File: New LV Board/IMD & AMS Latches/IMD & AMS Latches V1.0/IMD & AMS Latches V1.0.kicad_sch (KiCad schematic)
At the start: 21 parts, among them J2 B12B-PH-K-S, K1 A161CS12VDC.64, K2 A161CS12VDC.64, K3 A161CS12VDC.64, K4 A161CS12VDC.64, K5 A161CS12VDC.64, K6 A161CS12VDC.64, SW1 Test Reset IMD, SW2 Test Reset IMD

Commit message: added 3d models to the full part
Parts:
- D1, D2, D5, D6: footprint Diode_THT:D_DO-41_SOD81_P3.81mm_Vertical_AnodeUp -> motorsports:D_DO-41_SOD81_P3.81mm_Vertical_AnodeUp
- K1, K2, K3, K4, K5, K6: footprint Library:RELAY_A161CS12VDC.64 -> motorsports:RELAY_A161CS12VDC.64
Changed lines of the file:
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@@
 			)
 		)
-		(property "Footprint" "Library:RELAY_A161CS12VDC.64"
+		(property "Footprint" "motorsports:RELAY_A161CS12VDC.64"
 			(at 71.12 139.7 0)
 			(effects
@@
 			)
 		)
-		(property "Footprint" "Diode_THT:D_DO-41_SOD81_P3.81mm_Vertical_AnodeUp"
+		(property "Footprint" "motorsports:D_DO-41_SOD81_P3.81mm_Vertical_AnodeUp"
 			(at 133.35 147.32 0)
 			(effects
@@
 			)
 		)
-		(property "Footprint" "Library:RELAY_A161CS12VDC.64"
+		(property "Footprint" "motorsports:RELAY_A161CS12VDC.64"
 			(at 71.12 113.03 0)
 			(effects
@@
 			)
 		)
-		(property "Footprint" "Diode_THT:D_DO-41_SOD81_P3.81mm_Vertical_AnodeUp"
+		(property "Footprint" "motorsports:D_DO-41_SOD81_P3.81mm_Vertical_AnodeUp"
 			(at 50.8 147.32 0)
 			(effects
@@
 			)
 		)
-		(property "Footprint" "Diode_THT:D_DO-41_SOD81_P3.81mm_Vertical_AnodeUp"
+		(property "Footprint" "motorsports:D_DO-41_SOD81_P3.81mm_Vertical_AnodeUp"
 			(at 128.27 147.32 0)
 			(effects
@@
 			)
 		)
-		(property "Footprint" "Diode_THT:D_DO-41_SOD81_P3.81mm_Vertical_AnodeUp"
+		(property "Footprint" "motorsports:D_DO-41_SOD81_P3.81mm_Vertical_AnodeUp"
 			(at 55.88 147.32 0)
 			(effects
@@
 			)
 		)
-		(property "Footprint" "Library:RELAY_A161CS12VDC.64"
+		(property "Footprint" "motorsports:RELAY_A161CS12VDC.64"
 			(at 148.59 139.7 0)
 			(effects
@@
 			)
 		)
-		(property "Footprint" "Library:RELAY_A161CS12VDC.64"
+		(property "Footprint" "motorsports:RELAY_A161CS12VDC.64"
 			(at 148.59 113.03 0)
 			(effects
@@
 			)
 		)
-		(property "Footprint" "Library:RELAY_A161CS12VDC.64"
+		(property "Footprint" "motorsports:RELAY_A161CS12VDC.64"
 			(at 148.59 86.36 0)
 			(effects
@@
 			)
 		)
-		(property "Footprint" "Library:RELAY_A161CS12VDC.64"
+		(property "Footprint" "motorsports:RELAY_A161CS12VDC.64"
 			(at 71.12 86.36 0)
 			(effects

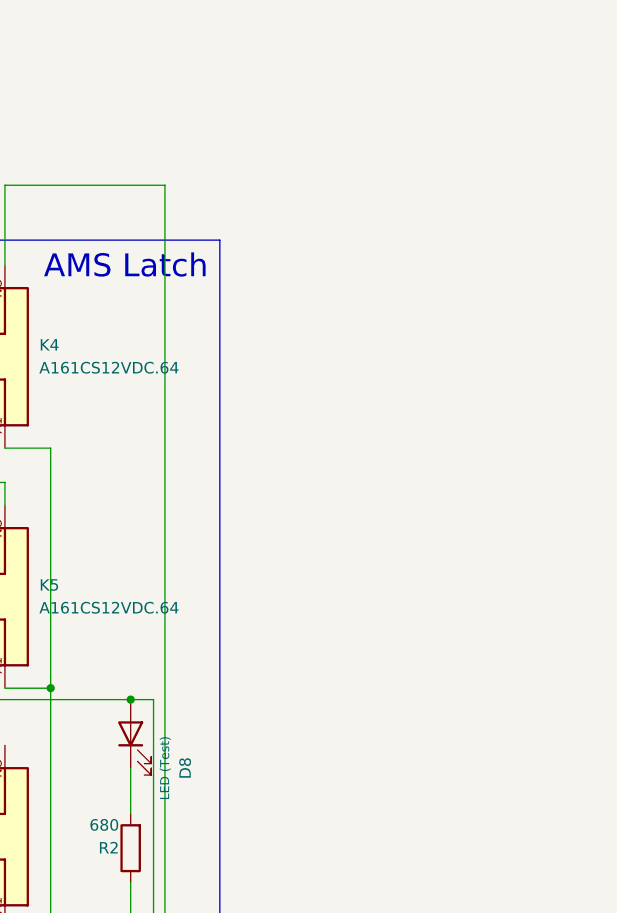
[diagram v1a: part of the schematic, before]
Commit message: changes that can probably be overriden?
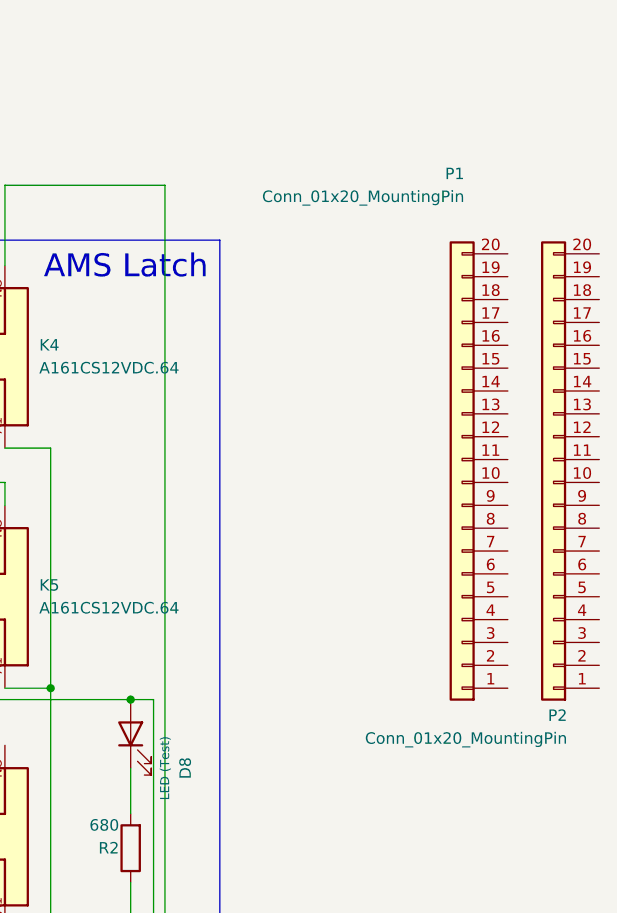
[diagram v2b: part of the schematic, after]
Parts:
- added P1, P2: Conn_01x20_MountingPin, Connector_PinHeader_2.54mm:PinHeader_1x20_P2.54mm_Vertical, symbol Connector_Generic:Conn_01x20
- D1, D2, D5, D6: Part # (none) -> 1N4743A
- D3, D7: Part # (none) -> 1N4001
- K1, K2, K3, K4, K5, K6: MANUFACTURER CIT -> (none); MAXIMUM_PACKAGE_HEIGHT 13.85mm -> (none); PARTREV B -> (none); SNAPEDA_PN A161CS12VDC.64 -> (none); STANDARD Manufacturer Recommendations -> (none)

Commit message: Revert "changes that can probably be overriden?"
This reverts commit 98343f344ad0564068fa41cd25b8ec5d82cca4ea.
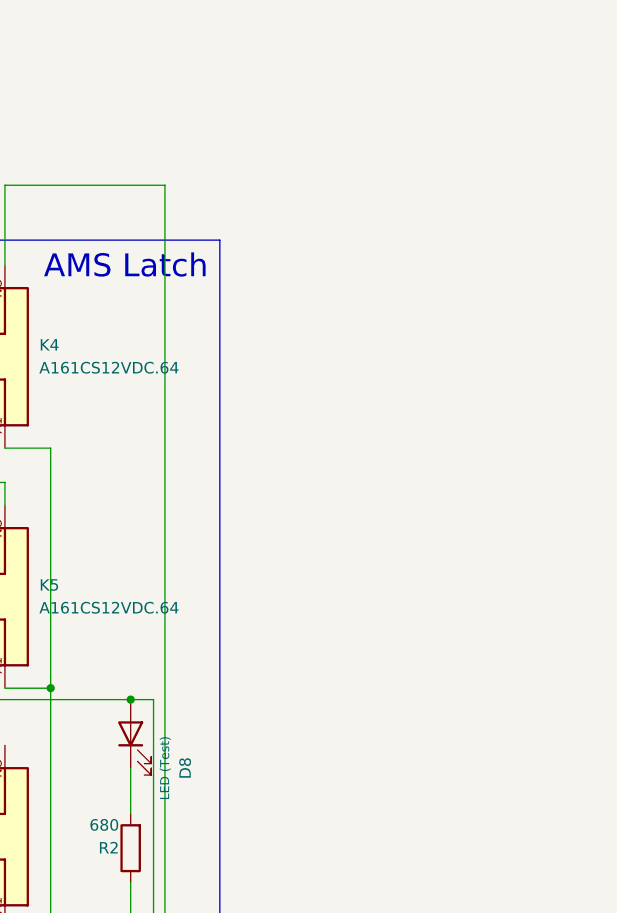
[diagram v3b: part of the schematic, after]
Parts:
- removed P1, P2: Conn_01x20_MountingPin, Connector_PinHeader_2.54mm:PinHeader_1x20_P2.54mm_Vertical, symbol Connector_Generic:Conn_01x20
- D1, D2, D5, D6: Part # 1N4743A -> (none)
- D3, D7: Part # 1N4001 -> (none)
- K1, K2, K3, K4, K5, K6: MANUFACTURER (none) -> CIT; MAXIMUM_PACKAGE_HEIGHT (none) -> 13.85mm; PARTREV (none) -> B; SNAPEDA_PN (none) -> A161CS12VDC.64; STANDARD (none) -> Manufacturer Recommendations
